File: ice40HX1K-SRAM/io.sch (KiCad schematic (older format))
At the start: 9 parts, among them J3 Conn_01x20_Male

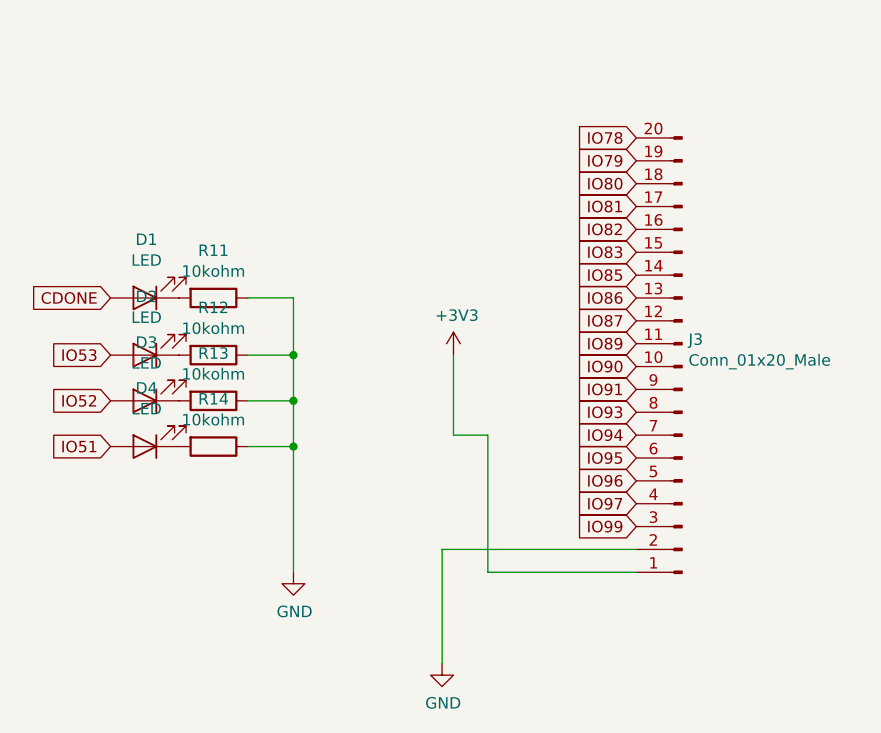
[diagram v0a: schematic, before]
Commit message: wiring FPGA
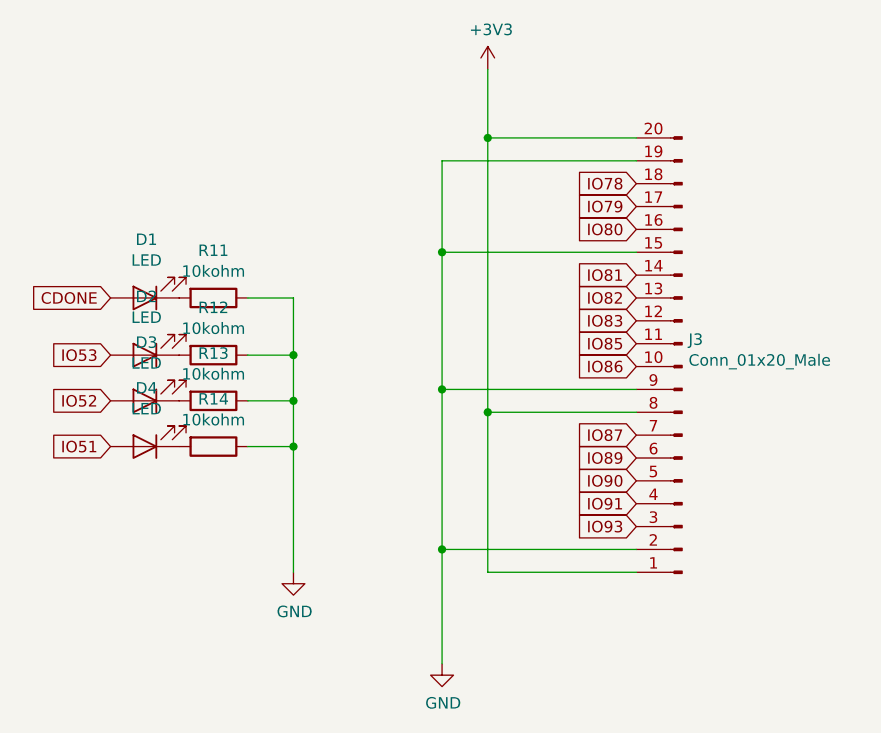
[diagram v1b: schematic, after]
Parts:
- R11, R12, R13, R14: footprint Resistor_SMD:R_1206_3216Metric -> Resistor_SMD:R_0402_1005Metric
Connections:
- net IO94 is gone; now on net IO87: J3.7 (Pin_7)
- net IO95 is gone; now on net IO89: J3.6 (Pin_6)
- net IO96 is gone; now on net IO90: J3.5 (Pin_5)
- net IO97 is gone; now on net IO91: J3.4 (Pin_4)
- net IO99 is gone; now on net IO93: J3.3 (Pin_3)
- net +3V3: now also J3.20 (Pin_20), J3.8 (Pin_8)
- net GND: now also J3.15 (Pin_15), J3.19 (Pin_19), J3.9 (Pin_9)
- net IO78: now also J3.18 (Pin_18); no longer J3.20 (Pin_20)
- net IO79: now also J3.17 (Pin_17); no longer J3.19 (Pin_19)
- net IO80: now also J3.16 (Pin_16); no longer J3.18 (Pin_18)
- net IO81: now also J3.14 (Pin_14); no longer J3.17 (Pin_17)
- net IO82: now also J3.13 (Pin_13); no longer J3.16 (Pin_16)
- net IO83: now also J3.12 (Pin_12); no longer J3.15 (Pin_15)
- net IO85: now also J3.11 (Pin_11); no longer J3.14 (Pin_14)
- net IO86: now also J3.10 (Pin_10); no longer J3.13 (Pin_13)
- net IO87: no longer J3.12 (Pin_12)
- net IO89: no longer J3.11 (Pin_11)
- net IO90: no longer J3.10 (Pin_10)
- net IO91: no longer J3.9 (Pin_9)
- net IO93: no longer J3.8 (Pin_8)
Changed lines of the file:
@@
 F 0 "R11" V 2993 3000 50  0000 C CNN
 F 1 "10kohm" V 3084 3000 50  0000 C CNN
-F 2 "Resistor_SMD:R_1206_3216Metric" V 3130 3000 50  0001 C CNN
+F 2 "Resistor_SMD:R_0402_1005Metric" V 3130 3000 50  0001 C CNN
 F 3 "~" H 3200 3000 50  0001 C CNN
 	1    3200 3000
@@
 F 0 "R12" V 2993 3250 50  0000 C CNN
 F 1 "10kohm" V 3084 3250 50  0000 C CNN
-F 2 "Resistor_SMD:R_1206_3216Metric" V 3130 3250 50  0001 C CNN
+F 2 "Resistor_SMD:R_0402_1005Metric" V 3130 3250 50  0001 C CNN
 F 3 "~" H 3200 3250 50  0001 C CNN
 	1    3200 3250
@@
 F 0 "R13" V 2993 3450 50  0000 C CNN
 F 1 "10kohm" V 3084 3450 50  0000 C CNN
-F 2 "Resistor_SMD:R_1206_3216Metric" V 3130 3450 50  0001 C CNN
+F 2 "Resistor_SMD:R_0402_1005Metric" V 3130 3450 50  0001 C CNN
 F 3 "~" H 3200 3450 50  0001 C CNN
 	1    3200 3450
@@
 F 0 "R14" V 2993 3650 50  0000 C CNN
 F 1 "10kohm" V 3084 3650 50  0000 C CNN
-F 2 "Resistor_SMD:R_1206_3216Metric" V 3130 3650 50  0001 C CNN
+F 2 "Resistor_SMD:R_0402_1005Metric" V 3130 3650 50  0001 C CNN
 F 3 "~" H 3200 3650 50  0001 C CNN
 	1    3200 3650
@@
 	3550 3650 3550 3450
 Connection ~ 3550 3450
-Text GLabel 5050 2300 0    50   Input ~ 0
+Text GLabel 5050 2500 0    50   Input ~ 0
 IO78
-Text GLabel 5050 2400 0    50   Input ~ 0
+Text GLabel 5050 2600 0    50   Input ~ 0
 IO79
-Text GLabel 5050 2500 0    50   Input ~ 0
+Text GLabel 5050 2700 0    50   Input ~ 0
 IO80
-Text GLabel 5050 2600 0    50   Input ~ 0
+Text GLabel 5050 2900 0    50   Input ~ 0
 IO81
-Text GLabel 5050 2700 0    50   Input ~ 0
+Text GLabel 5050 3000 0    50   Input ~ 0
 IO82
-Text GLabel 5050 2800 0    50   Input ~ 0
+Text GLabel 5050 3100 0    50   Input ~ 0
 IO83
-Text GLabel 5050 2900 0    50   Input ~ 0
+Text GLabel 5050 3200 0    50   Input ~ 0
 IO85
-Text GLabel 5050 3000 0    50   Input ~ 0
+Text GLabel 5050 3300 0    50   Input ~ 0
 IO86
-Text GLabel 5050 3100 0    50   Input ~ 0
+Text GLabel 5050 3600 0    50   Input ~ 0
 IO87
-Text GLabel 5050 3200 0    50   Input ~ 0
+Text GLabel 5050 3700 0    50   Input ~ 0
 IO89
-Text GLabel 5050 3300 0    50   Input ~ 0
+Text GLabel 5050 3800 0    50   Input ~ 0
 IO90
-Text GLabel 5050 3400 0    50   Input ~ 0
+Text GLabel 5050 3900 0    50   Input ~ 0
 IO91
-Text GLabel 5050 3500 0    50   Input ~ 0
+Text GLabel 5050 4000 0    50   Input ~ 0
 IO93
-Text GLabel 5050 3600 0    50   Input ~ 0
-IO94
-Text GLabel 5050 3700 0    50   Input ~ 0
-IO95
-Text GLabel 5050 3800 0    50   Input ~ 0
-IO96
-Text GLabel 5050 3900 0    50   Input ~ 0
-IO97
-Text GLabel 5050 4000 0    50   Input ~ 0
-IO99
 $Comp
 L Connector:Conn_01x20_Male J3
@@
 L power:+3V3 #PWR099
 U 1 1 5E64C825
-P 4250 3250
-F 0 "#PWR099" H 4250 3100 50  0001 C CNN
-F 1 "+3V3" H 4265 3423 50  0000 C CNN
-F 2 "" H 4250 3250 50  0001 C CNN
-F 3 "" H 4250 3250 50  0001 C CNN
-	1    4250 3250
+P 4400 2000
+F 0 "#PWR099" H 4400 1850 50  0001 C CNN
+F 1 "+3V3" H 4415 2173 50  0000 C CNN
+F 2 "" H 4400 2000 50  0001 C CNN
+F 3 "" H 4400 2000 50  0001 C CNN
+	1    4400 2000
 	1    0    0    -1
 $EndComp
@@
 	5050 4200 4400 4200
 Wire Wire Line
-	4400 4200 4400 3600
-Wire Wire Line
-	4400 3600 4250 3600
-Wire Wire Line
-	4250 3600 4250 3250
+	4400 2000 4400 2300
+Wire Wire Line
+	4400 3500 5050 3500
+Connection ~ 4400 3500
+Wire Wire Line
+	4400 3500 4400 4200
+Wire Wire Line
+	4200 4100 4200 3400
+Wire Wire Line
+	4200 3400 5050 3400
+Connection ~ 4200 4100
+Wire Wire Line
+	4200 2400 5050 2400
+Wire Wire Line
+	4400 2300 5050 2300
+Connection ~ 4400 2300
+Wire Wire Line
+	4400 2300 4400 3500
+Wire Wire Line
+	4200 2800 5050 2800
+Connection ~ 4200 2800
+Wire Wire Line
+	4200 2800 4200 2400
+Wire Wire Line
+	4200 2800 4200 3400
+Connection ~ 4200 3400
 $EndSCHEMATC
